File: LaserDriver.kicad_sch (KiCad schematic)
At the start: 27 parts, among them J100 Screw_Terminal_01x02, J102 Screw_Terminal_01x02, J103 Screw_Terminal_01x02, U1 TPS92513DGQR

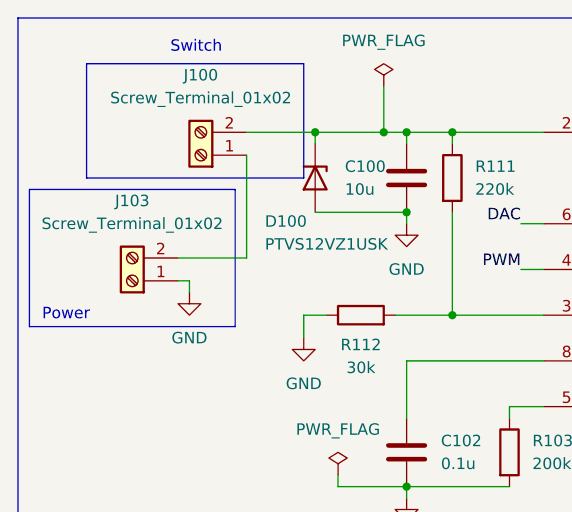
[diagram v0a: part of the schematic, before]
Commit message: compactified design
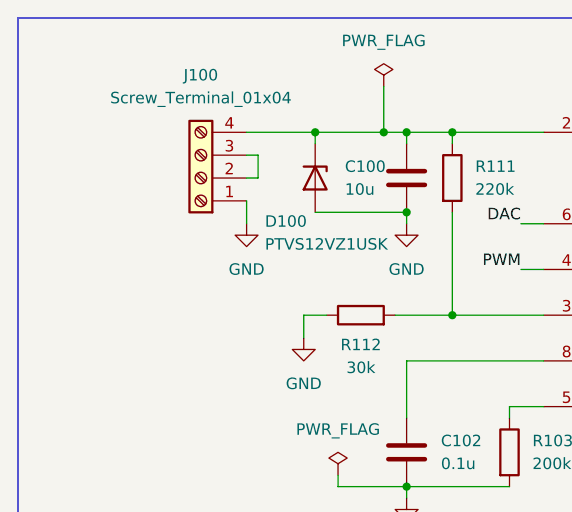
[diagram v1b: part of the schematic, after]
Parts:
- removed J100, J103: Screw_Terminal_01x02, TerminalBlock:TerminalBlock_MaiXu_MX126-5.0-02P_1x02_P5.00mm, symbol Connector:Screw_Terminal_01x02
- added J100: Screw_Terminal_01x04, TerminalBlock:TerminalBlock_MaiXu_MX126-5.0-04P_1x04_P5.00mm, symbol Connector:Screw_Terminal_01x04
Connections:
- net GND: now also J100.1 (Pin_1)
- net at C100.1, D100.1 (K), R111.1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: now also J100.4 (Pin_4)
- new net: J100.2 (Pin_2), J100.3 (Pin_3)
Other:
- note removed: "Power"
- note removed: "Switch"
